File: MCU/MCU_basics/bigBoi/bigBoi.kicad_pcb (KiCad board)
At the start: 2 copper layers, 62 x 62 mm, 86 parts, among them IC1 BMP390, J3 DM3AT-SF-PEJM5_40_, J4 Conn_01x05, J5 Conn_01x04, J6 Conn_01x06, J7 USB_B_Micro, SW1 Boot Switch, U1 STM32F469NIHx, U2 LT1963AxST-3.3, U3 SX1276, U5 MIA-M10Q, U6 BNO086, Y1 8MHz, Y3 32kHz

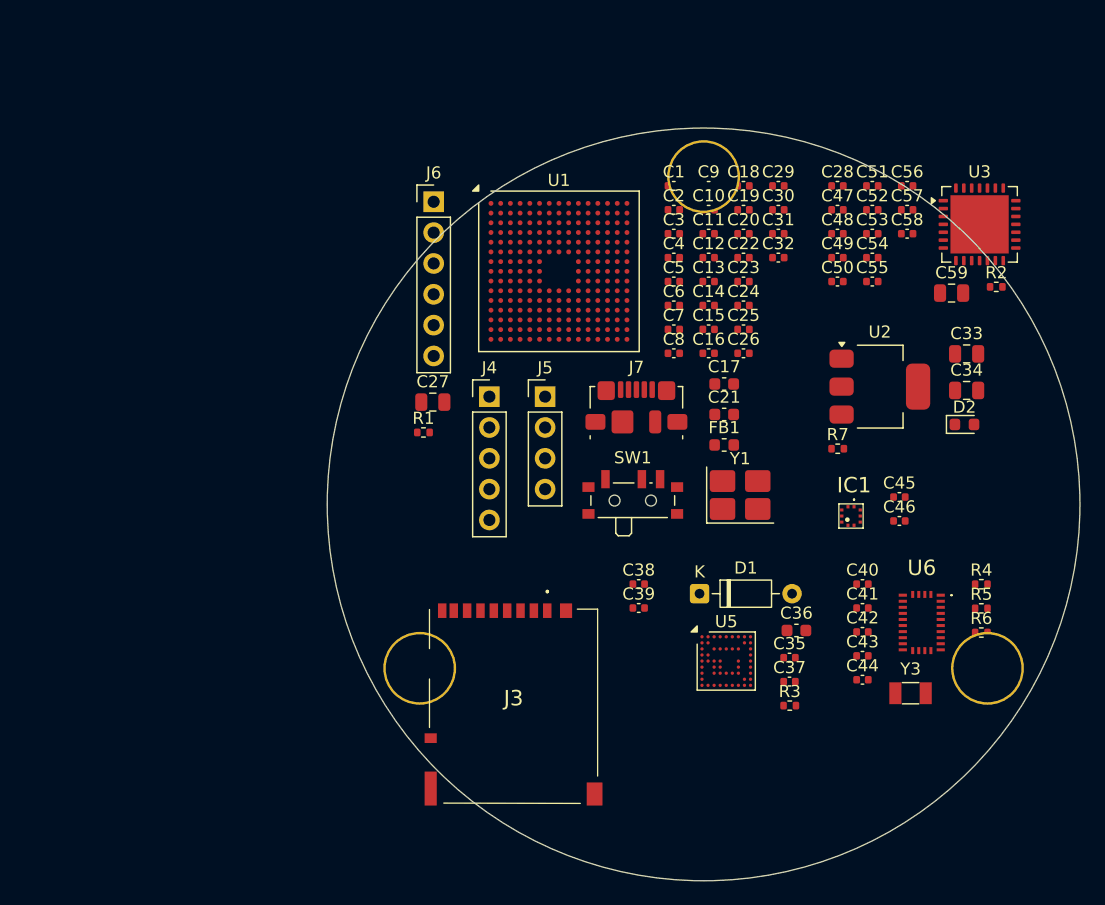
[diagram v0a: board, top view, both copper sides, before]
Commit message: update nebula FP
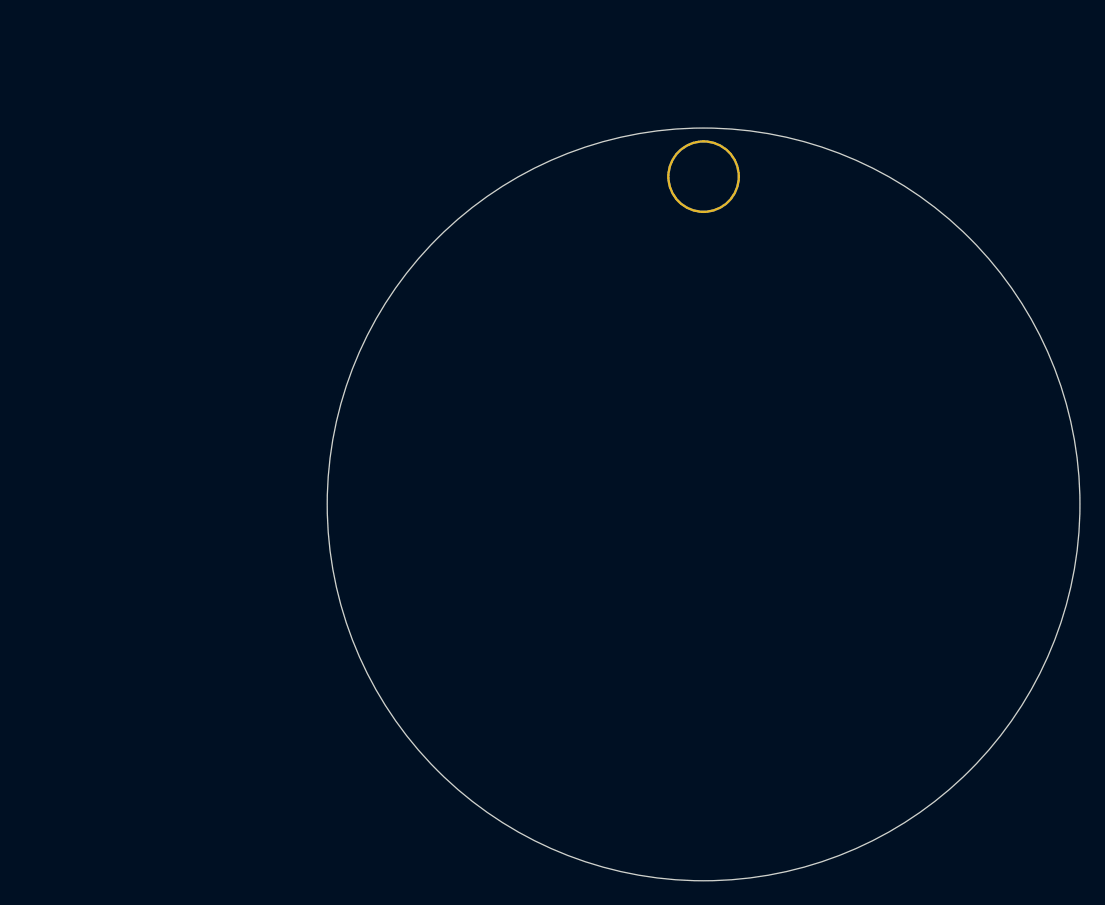
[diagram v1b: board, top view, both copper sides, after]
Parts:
- removed C1, C10, C12, C15, C16, C19, C2, C20, C22, C23, C24, C25, C26, C3, C30, C35, C37, C39, C4, C48, C49, C5, C50, C51, C52, C54, C6, C7, C8, C9: 100nF, Capacitor_SMD:C_0402_1005Metric
- removed C11: 10nF, Capacitor_SMD:C_0402_1005Metric
- removed C13, C29, C31, C32, C38: 1uF, Capacitor_SMD:C_0402_1005Metric
- removed C14, C18: 0402, Capacitor_SMD:C_0402_1005Metric
- removed C17, C21: 2.2uF, Capacitor_SMD:C_0603_1608Metric
- removed C27, C59: 10uF, Capacitor_SMD:C_0805_2012Metric
- removed C28, C47: 15pF, Capacitor_SMD:C_0402_1005Metric
- removed C33, C34: 22uF, Capacitor_SMD:C_0805_2012Metric
- removed C36: 10uF, Capacitor_SMD:C_0603_1608Metric
- removed C40, C41, C43: 0.1uF, Capacitor_SMD:C_0402_1005Metric
- removed C42: 22pF, Capacitor_SMD:C_0402_1005Metric
- removed C44: 22PF, Capacitor_SMD:C_0402_1005Metric
- removed C45, C46: 100nf, Capacitor_SMD:C_0402_1005Metric
- removed C53, C58: 47pF, Capacitor_SMD:C_0402_1005Metric
- removed C55: 1.5pF, Capacitor_SMD:C_0402_1005Metric
- removed C56: 4.7pF, Capacitor_SMD:C_0402_1005Metric
- removed C57: 1nF, Capacitor_SMD:C_0402_1005Metric
- removed D1: 1N914, Diode_THT:D_DO-35_SOD27_P7.62mm_Horizontal
- removed D2: GREEN, LED_SMD:LED_0603_1608Metric
- removed FB1: 120R, Inductor_SMD:L_0603_1608Metric
- removed IC1: BMP390, Nebula-footprints:BMP390
- removed J3: DM3AT-SF-PEJM5_40_, Nebula-footprints:DM3ATSFPEJM540
- removed J4: Conn_01x05, Connector_PinHeader_2.54mm:PinHeader_1x05_P2.54mm_Vertical
- removed J5: Conn_01x04, Connector_PinHeader_2.54mm:PinHeader_1x04_P2.54mm_Vertical
- removed J6: Conn_01x06, Connector_PinHeader_2.54mm:PinHeader_1x06_P2.54mm_Vertical
- removed J7: USB_B_Micro, Connector_USB:USB_Micro-B_Molex_47346-0001
- removed R1, R2, R3, R4: 10k, Resistor_SMD:R_0402_1005Metric
- removed R5, R6: 2.2k, Resistor_SMD:R_0402_1005Metric
- removed R7: 1k5, Resistor_SMD:R_0402_1005Metric
- removed the REF** at (152.3, 118.0)
- removed the REF** at (105.5, 118.0)
- removed SW1: Boot Switch, Button_Switch_SMD:SW_SPDT_PCM12
- removed U1: STM32F469NIHx, Package_BGA:TFBGA-216_13x13mm_Layout15x15_P0.8mm
- removed U2: LT1963AxST-3.3, Package_TO_SOT_SMD:SOT-223-3_TabPin2
- removed U3: SX1276, Package_DFN_QFN:QFN-28-1EP_6x6mm_P0.65mm_EP4.8x4.8mm
- removed U5: MIA-M10Q, Package_LGA:ublox_LGA-53_4.5x4.5mm_Layout9x9_P0.5mm
- removed U6: BNO086, Nebula-footprints:BNO086
- removed Y1: 8MHz, Crystal:Crystal_SMD_3225-4Pin_3.2x2.5mm_HandSoldering
- removed Y3: 32kHz, Crystal:Crystal_SMD_3215-2Pin_3.2x1.5mm

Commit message: Bat
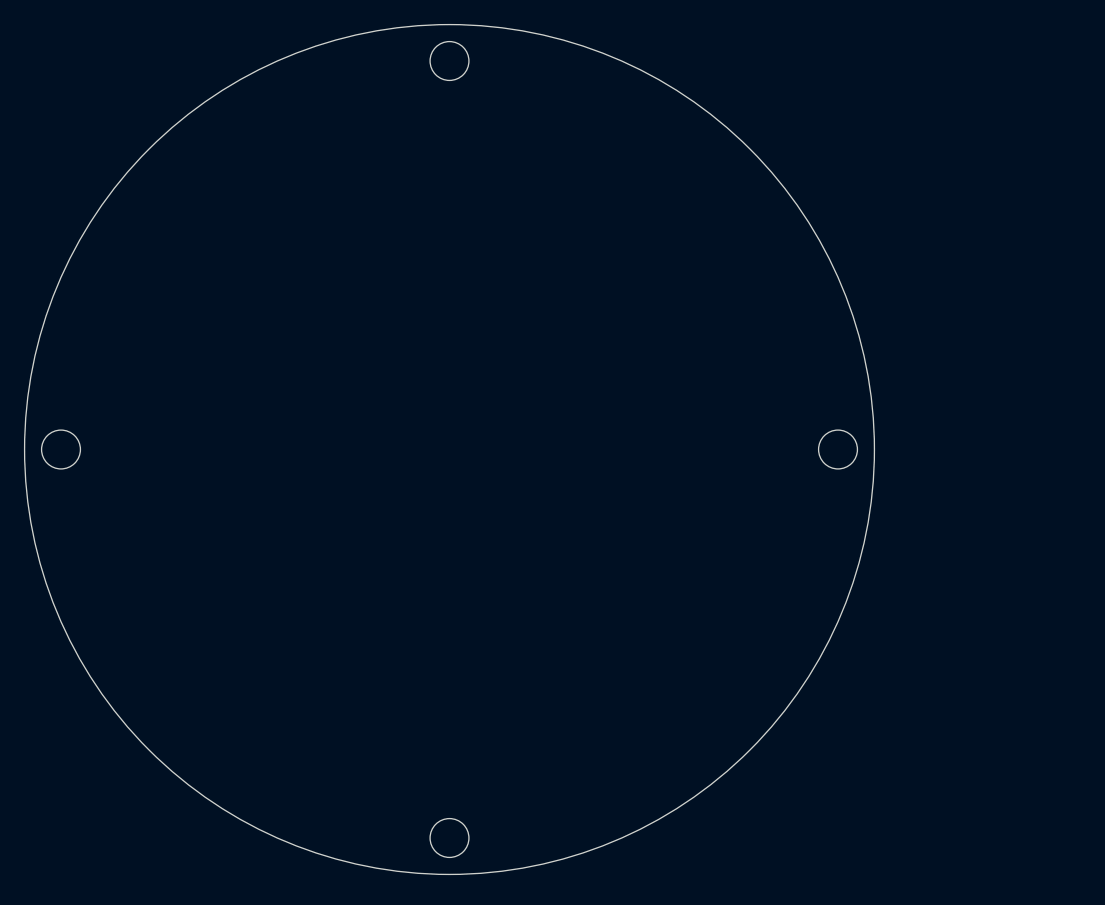
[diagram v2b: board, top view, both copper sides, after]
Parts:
- removed the REF** at (128.9, 77.5)
- added REF**: MountingHole_3.2mm_M3, MountingHole:MountingHole_3.2mm_M3, F.Cu at (140.0, 100.0)
- added REF**: MountingHole_3.2mm_M3, MountingHole:MountingHole_3.2mm_M3, F.Cu at (108.0, 132.0)
- added REF**: MountingHole_3.2mm_M3, MountingHole:MountingHole_3.2mm_M3, F.Cu at (108.0, 68.0)
- added REF**: MountingHole_3.2mm_M3, MountingHole:MountingHole_3.2mm_M3, F.Cu at (76.0, 100.0)
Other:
- board size 62 x 62 mm -> 70 x 70 mm
